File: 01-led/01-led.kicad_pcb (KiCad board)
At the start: 2 copper layers, 12.7 x 16.5 mm, 4 parts, among them J1 Conn_01x02_Socket, J2 Conn_01x02_Socket

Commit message: update pcb
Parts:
- D1, D2: footprint LED_THT:LED_D3.0mm -> Library:LED_THT__LED_D3.0mm
- J1, J2: footprint Connector_PinSocket_2.54mm:PinSocket_1x02_P2.54mm_Vertical -> Library:Connector__PinSocket_1x02_P2.54mm_Vertical
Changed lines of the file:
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@@
   (net 2 "Net-(D1-A)")
   (net 3 "Net-(D2-A)")
-  (footprint "LED_THT:LED_D3.0mm" (layer "F.Cu")
+  (footprint "Library:LED_THT__LED_D3.0mm" (layer "F.Cu")
     (at 132.08 87.63 90)
     (descr "LED, diameter 3.0mm, 2 pins")
@@
     )
   )
-  (footprint "LED_THT:LED_D3.0mm" (layer "F.Cu")
+  (footprint "Library:LED_THT__LED_D3.0mm" (layer "F.Cu")
     (at 137.16 87.63 90)
     (descr "LED, diameter 3.0mm, 2 pins")
@@
     )
   )
-  (footprint "Connector_PinSocket_2.54mm:PinSocket_1x02_P2.54mm_Vertical" (layer "B.Cu")
+  (footprint "Library:Connector__PinSocket_1x02_P2.54mm_Vertical" (layer "B.Cu")
     (at 132.08 91.44 -90)
     (descr "Through hole straight socket strip, 1x02, 2.54mm pitch, single row (from Kicad 4.0.7), script generated")
@@
         (effects (font (size 1 1) (thickness 0.15)) (justify mirror))
     )
-    (fp_text user "${REFERENCE}" (at 0 -1.27) (layer "B.Fab")
+    (fp_text user "${REFERENCE}" (at 0 -1.27 180) (layer "B.Fab")
         (effects (font (size 1 1) (thickness 0.15)) (justify mirror))
     )
@@
     )
   )
-  (footprint "Connector_PinSocket_2.54mm:PinSocket_1x02_P2.54mm_Vertical" (layer "B.Cu")
+  (footprint "Library:Connector__PinSocket_1x02_P2.54mm_Vertical" (layer "B.Cu")
     (at 132.08 96.52 -90)
     (descr "Through hole straight socket strip, 1x02, 2.54mm pitch, single row (from Kicad 4.0.7), script generated")
@@
         (effects (font (size 1 1) (thickness 0.15)) (justify mirror))
     )
-    (fp_text user "${REFERENCE}" (at 0 -1.27) (layer "B.Fab")
-        (effects (font (size 1 1) (thickness 0.15)) (justify mirror))
-    )
+    (fp_text user "${REFERENCE}" (at 0 -1.27 180) (layer "B.Fab")
+        (effects (font (size 1 1) (thickness 0.15)) (justify mirror))
+    )

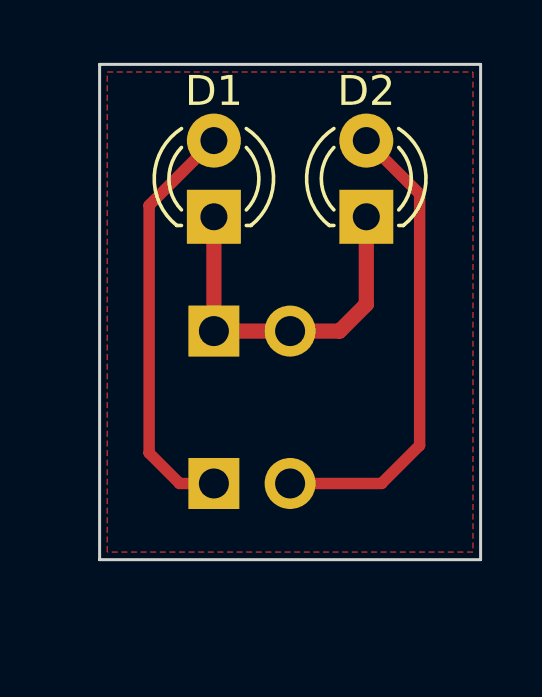
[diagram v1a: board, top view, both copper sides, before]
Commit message: update pcb
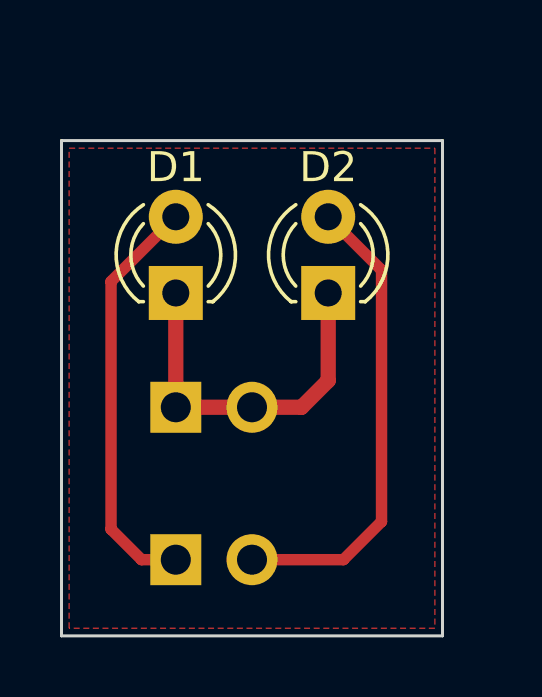
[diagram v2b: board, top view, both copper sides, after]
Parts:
- moved D1 2.84 mm to (130.8, 90.2)
- moved D2 2.84 mm to (135.9, 90.2)
- moved J1 2.84 mm to (130.8, 99.1)
- moved J2 2.84 mm to (130.8, 94.0)
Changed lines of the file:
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@@
   (setup
     (pad_to_mask_clearance 0)
+    (aux_axis_origin 127 101.6)
+    (grid_origin 127 101.6)
     (pcbplotparams
       (layerselection 0x00010fc_ffffffff)
@@
   (net 3 "Net-(D2-A)")
   (footprint "Library:LED_THT__LED_D3.0mm" (layer "F.Cu")
-    (at 132.08 87.63 90)
+    (at 130.81 90.17 90)
     (descr "LED, diameter 3.0mm, 2 pins")
     (tags "LED diameter 3.0mm 2 pins")
@@
   )
   (footprint "Library:LED_THT__LED_D3.0mm" (layer "F.Cu")
-    (at 137.16 87.63 90)
+    (at 135.89 90.17 90)
     (descr "LED, diameter 3.0mm, 2 pins")
     (tags "LED diameter 3.0mm 2 pins")
@@
   )
   (footprint "Library:Connector__PinSocket_1x02_P2.54mm_Vertical" (layer "B.Cu")
-    (at 132.08 91.44 -90)
+    (at 130.81 93.98 -90)
     (descr "Through hole straight socket strip, 1x02, 2.54mm pitch, single row (from Kicad 4.0.7), script generated")
     (tags "Through hole socket strip THT 1x02 2.54mm single row")
@@
   )
   (footprint "Library:Connector__PinSocket_1x02_P2.54mm_Vertical" (layer "B.Cu")
-    (at 132.08 96.52 -90)
+    (at 130.81 99.06 -90)
     (descr "Through hole straight socket strip, 1x02, 2.54mm pitch, single row (from Kicad 4.0.7), script generated")
     (tags "Through hole socket strip THT 1x02 2.54mm single row")
@@
     )
   )
-  (gr_line (start 128.27 99.06) (end 128.27 82.55)
+  (gr_line (start 127 101.6) (end 127 85.09)
     (stroke (width 0.1) (type default)) (layer "Edge.Cuts"))
-  (gr_line (start 140.97 82.55) (end 140.97 99.06)
+  (gr_line (start 139.7 85.09) (end 139.7 101.6)
     (stroke (width 0.1) (type default)) (layer "Edge.Cuts"))
-  (gr_line (start 128.27 82.55) (end 140.97 82.55)
+  (gr_line (start 127 85.09) (end 139.7 85.09)
     (stroke (width 0.1) (type default)) (layer "Edge.Cuts"))
-  (gr_line (start 140.97 99.06) (end 128.27 99.06)
+  (gr_line (start 139.7 101.6) (end 127 101.6)
     (stroke (width 0.1) (type default)) (layer "Edge.Cuts"))
-  (segment (start 132.08 91.44) (end 134.62 91.44) (width 0.508) (layer "F.Cu") (net 1))
-  (segment (start 137.16 90.551) (end 137.16 87.63) (width 0.508) (layer "F.Cu") (net 1))
-  (segment (start 136.271 91.44) (end 137.16 90.551) (width 0.508) (layer "F.Cu") (net 1))
-  (segment (start 134.62 91.44) (end 136.271 91.44) (width 0.508) (layer "F.Cu") (net 1))
-  (segment (start 132.08 87.63) (end 132.08 91.44) (width 0.508) (layer "F.Cu") (net 1))
-  (segment (start 129.921 95.504) (end 129.921 87.249) (width 0.381) (layer "F.Cu") (net 2))
-  (segment (start 130.937 96.52) (end 129.921 95.504) (width 0.381) (layer "F.Cu") (net 2))
-  (segment (start 129.921 87.249) (end 132.08 85.09) (width 0.381) (layer "F.Cu") (net 2))
-  (segment (start 132.08 96.52) (end 130.937 96.52) (width 0.381) (layer "F.Cu") (net 2))
-  (segment (start 137.668 96.52) (end 138.938 95.25) (width 0.381) (layer "F.Cu") (net 3))
-  (segment (start 138.938 95.25) (end 138.938 86.868) (width 0.381) (layer "F.Cu") (net 3))
-  (segment (start 138.938 86.868) (end 137.16 85.09) (width 0.381) (layer "F.Cu") (net 3))
-  (segment (start 134.62 96.52) (end 137.668 96.52) (width 0.381) (layer "F.Cu") (net 3))
+  (segment (start 130.81 93.98) (end 133.35 93.98) (width 0.508) (layer "F.Cu") (net 1))
+  (segment (start 135.89 93.091) (end 135.89 90.17) (width 0.508) (layer "F.Cu") (net 1))
+  (segment (start 135.001 93.98) (end 135.89 93.091) (width 0.508) (layer "F.Cu") (net 1))
+  (segment (start 133.35 93.98) (end 135.001 93.98) (width 0.508) (layer "F.Cu") (net 1))
+  (segment (start 130.81 90.17) (end 130.81 93.98) (width 0.508) (layer "F.Cu") (net 1))
+  (segment (start 128.651 98.044) (end 128.651 89.789) (width 0.381) (layer "F.Cu") (net 2))
+  (segment (start 129.667 99.06) (end 128.651 98.044) (width 0.381) (layer "F.Cu") (net 2))
+  (segment (start 128.651 89.789) (end 130.81 87.63) (width 0.381) (layer "F.Cu") (net 2))
+  (segment (start 130.81 99.06) (end 129.667 99.06) (width 0.381) (layer "F.Cu") (net 2))
+  (segment (start 136.398 99.06) (end 137.668 97.79) (width 0.381) (layer "F.Cu") (net 3))
+  (segment (start 137.668 97.79) (end 137.668 89.408) (width 0.381) (layer "F.Cu") (net 3))
+  (segment (start 137.668 89.408) (end 135.89 87.63) (width 0.381) (layer "F.Cu") (net 3))
+  (segment (start 133.35 99.06) (end 136.398 99.06) (width 0.381) (layer "F.Cu") (net 3))
   (zone (net 1) (net_name "GND") (layer "F.Cu") (hatch edge 0.5)
     (connect_pads (clearance 0.5))
@@
     (polygon
       (pts
-        (xy 128.524 82.804)
-        (xy 140.716 82.804)
-        (xy 140.716 98.806)
-        (xy 128.524 98.806)
+        (xy 127.254 85.344)
+        (xy 139.446 85.344)
+        (xy 139.446 101.346)
+        (xy 127.254 101.346)
       )
     )
